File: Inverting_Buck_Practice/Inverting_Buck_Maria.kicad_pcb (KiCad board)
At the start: 2 copper layers, 11 parts, among them J1 Screw_Terminal_2x5.08, J2 Screw_Terminal_2x5.08, U1 MC33063AD

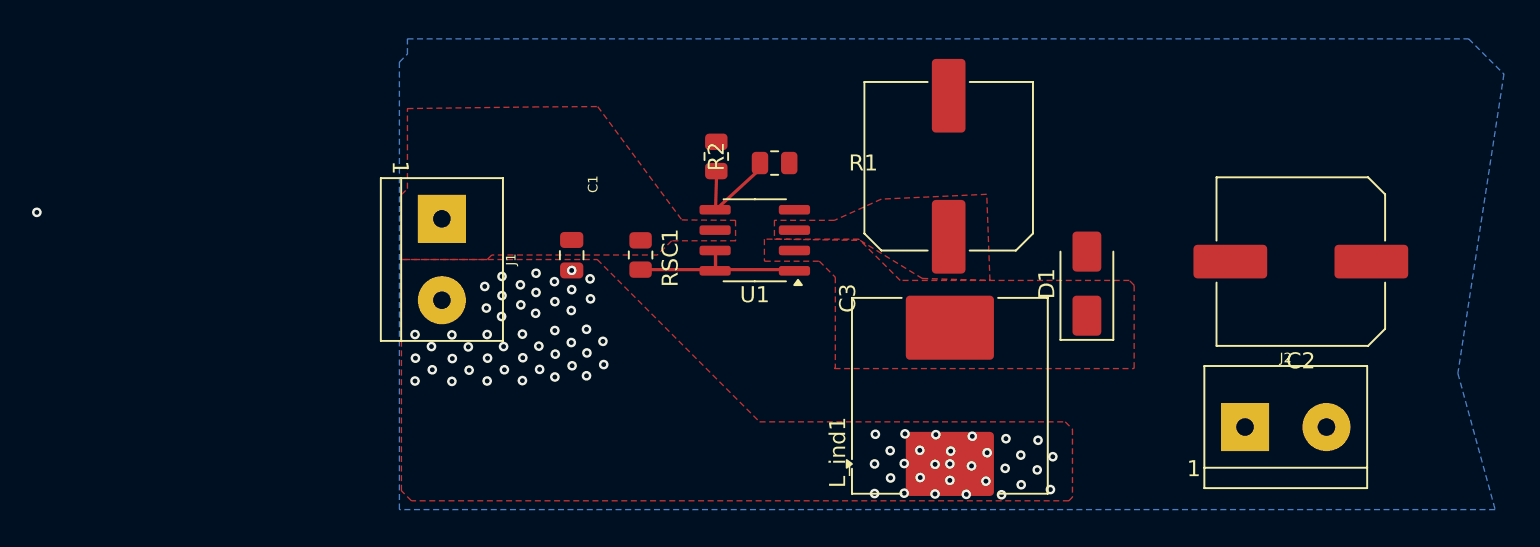
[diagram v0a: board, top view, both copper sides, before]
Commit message: Finishing another draft of Inverting Buck
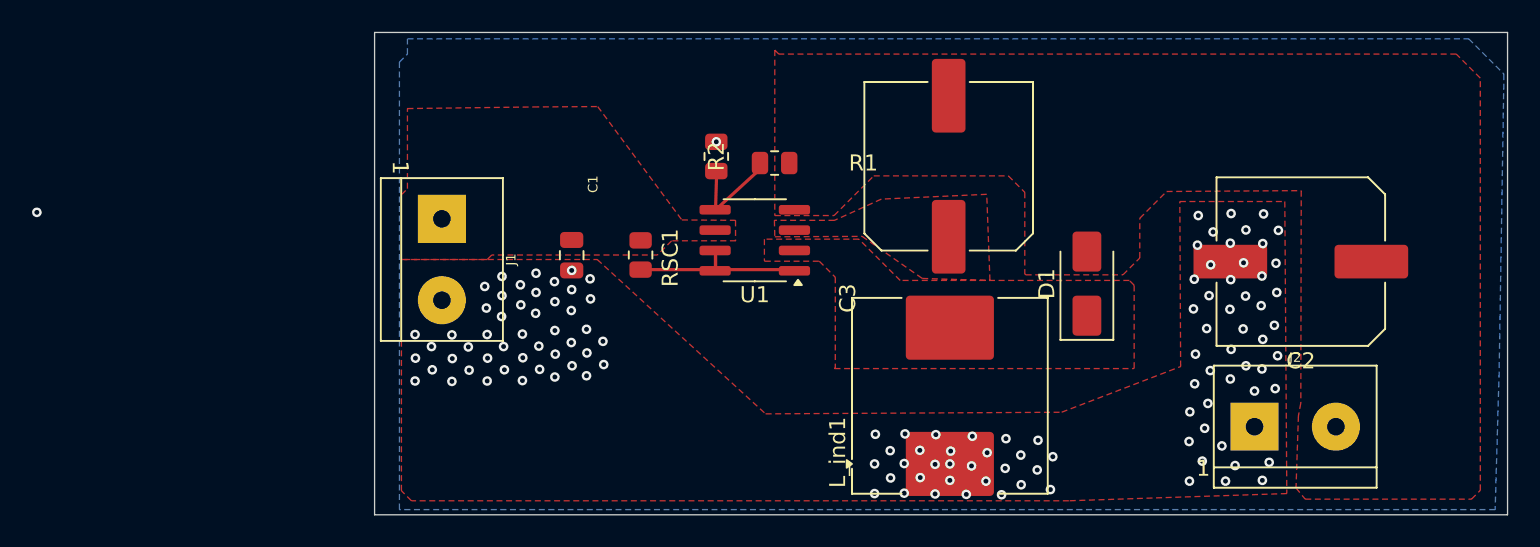
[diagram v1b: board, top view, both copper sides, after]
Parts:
- moved J2 0.59 mm to (153.8, 149.3)
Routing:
- net GND: vias 77 -> 124
- added copper zone on F.Cu, net /V_out
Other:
- board outline added: 70.7 x 30.1 mm
